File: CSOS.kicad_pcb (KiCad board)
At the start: 2 copper layers, 42 x 57 mm, 27 parts, among them P101 CONN_01X02, P102 CONN_01X03, P103 CONN_01X02, P201 CONN_01X01, Q201 Q_NMOS_GDS, U201 LMV358, U401 LM2931D-R

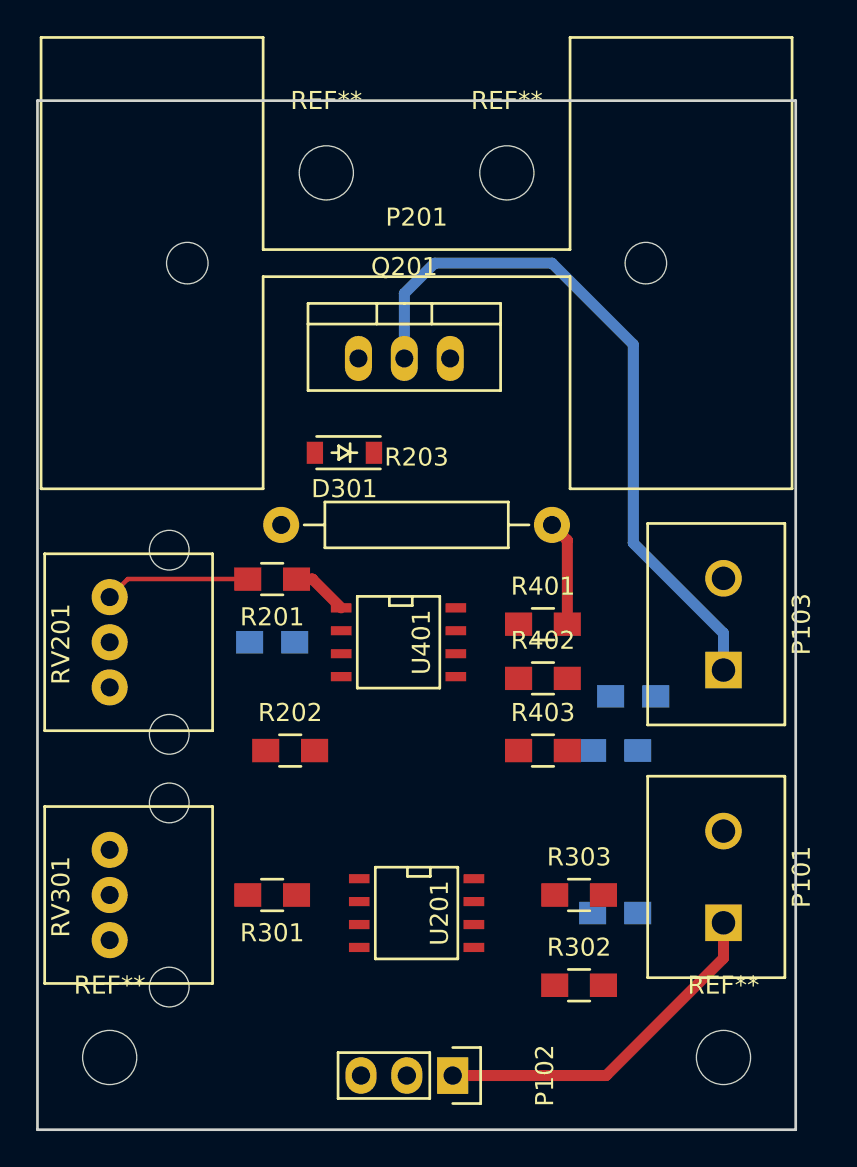
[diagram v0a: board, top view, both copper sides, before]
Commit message: Layout connected.
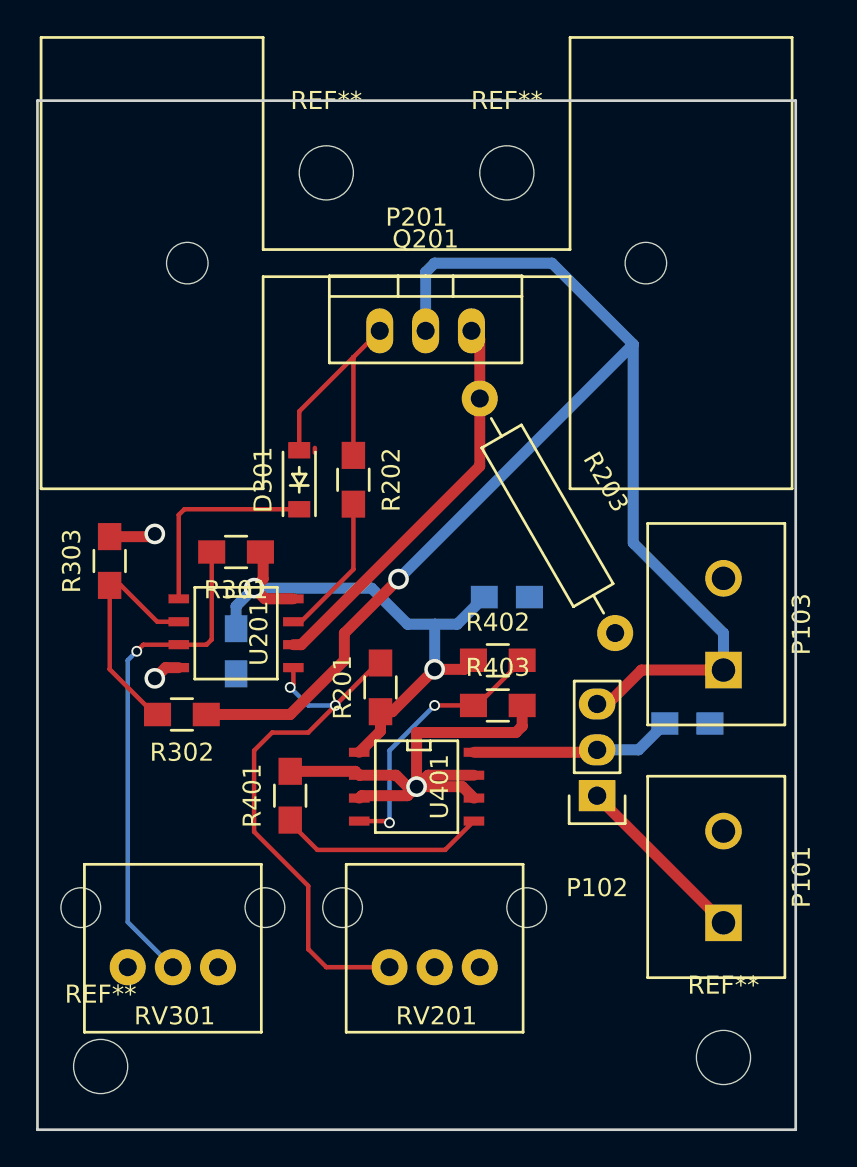
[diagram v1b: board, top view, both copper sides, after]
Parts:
- removed C301: C, Capacitors_SMD:C_0805_HandSoldering
- moved R303 31.9 mm to (131.0, 92.5), turned to 90 degrees
- moved R302 26.6 mm to (135.0, 101.0), turned to 180 degrees
- moved RV201 25.5 mm to (149.0, 115.0), turned to 0 degrees
- moved R301 19.1 mm to (138.0, 92.0)
- moved U201 18.4 mm to (138.0, 96.5)
- moved P102 17.4 mm to (158.0, 105.5), turned to 180 degrees
- moved R401 16.9 mm to (141.0, 105.5), turned to 90 degrees
- moved R202 15.4 mm to (144.5, 88.0), turned to 270 degrees
- moved R203 13.0 mm to (151.5, 83.5), turned to 300 degrees
- moved C402 8.90 mm to (153.0, 94.5)
- moved R201 8.49 mm to (146.0, 99.5), turned to 90 degrees
- moved U401 8.06 mm to (148.0, 105.0)
- moved RV301 5.32 mm to (134.5, 115.0), turned to 0 degrees
- moved C401 4.27 mm to (163.0, 101.5)
- moved R403 3.54 mm to (152.5, 100.5)
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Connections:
- U201 pad 1: Net-(R202-Pad2) -> Net-(D301-Pad1)
- U201 pad 2: Net-(Q201-Pad3) -> Net-(R302-Pad2)
- U201 pad 3: Net-(R201-Pad2) -> Net-(R301-Pad2)
- U201 pad 5: Net-(R301-Pad2) -> Net-(R201-Pad2)
- U201 pad 6: Net-(R302-Pad2) -> Net-(Q201-Pad3)
- U201 pad 7: Net-(D301-Pad1) -> Net-(R202-Pad2)
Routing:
- net /Current Control/Current_Sink+: track 39.0 -> 77.7 mm, vias 0 -> 1
- net 2.7V: track 3.14 -> 33.1 mm, vias 0 -> 2
- net Net-(R301-Pad2): track 0.00 -> 28.0 mm, vias 0 -> 1
- net GND: track 5.85 -> 31.9 mm, vias 0 -> 3
- net Net-(R201-Pad2): track 8.06 -> 30.2 mm, vias 0 -> 2
- net Net-(Q201-Pad3): track 0.00 -> 22.1 mm
- net Net-(R402-Pad2): track 0.00 -> 15.1 mm, vias 0 -> 2
- net /Current Control/FET_Gate: track 0.27 -> 14.0 mm
- net Net-(R302-Pad2): track 0.00 -> 13.0 mm
- net Net-(R401-Pad1): track 0.00 -> 11.6 mm
- net Net-(D301-Pad1): track 0.00 -> 11.5 mm
- net /Power Regulation/Vin: track 0.00 -> 11.2 mm
- net Net-(P101-Pad1): track 19.7 -> 9.98 mm
- net Net-(R202-Pad2): track 0.00 -> 8.14 mm
